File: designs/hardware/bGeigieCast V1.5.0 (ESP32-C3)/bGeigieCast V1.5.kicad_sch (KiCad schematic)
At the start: 9 parts, among them SW1 TACT-SWITCH, SW2 SWITCH_INV, U1 ESP32S, U2 XBEE-socket

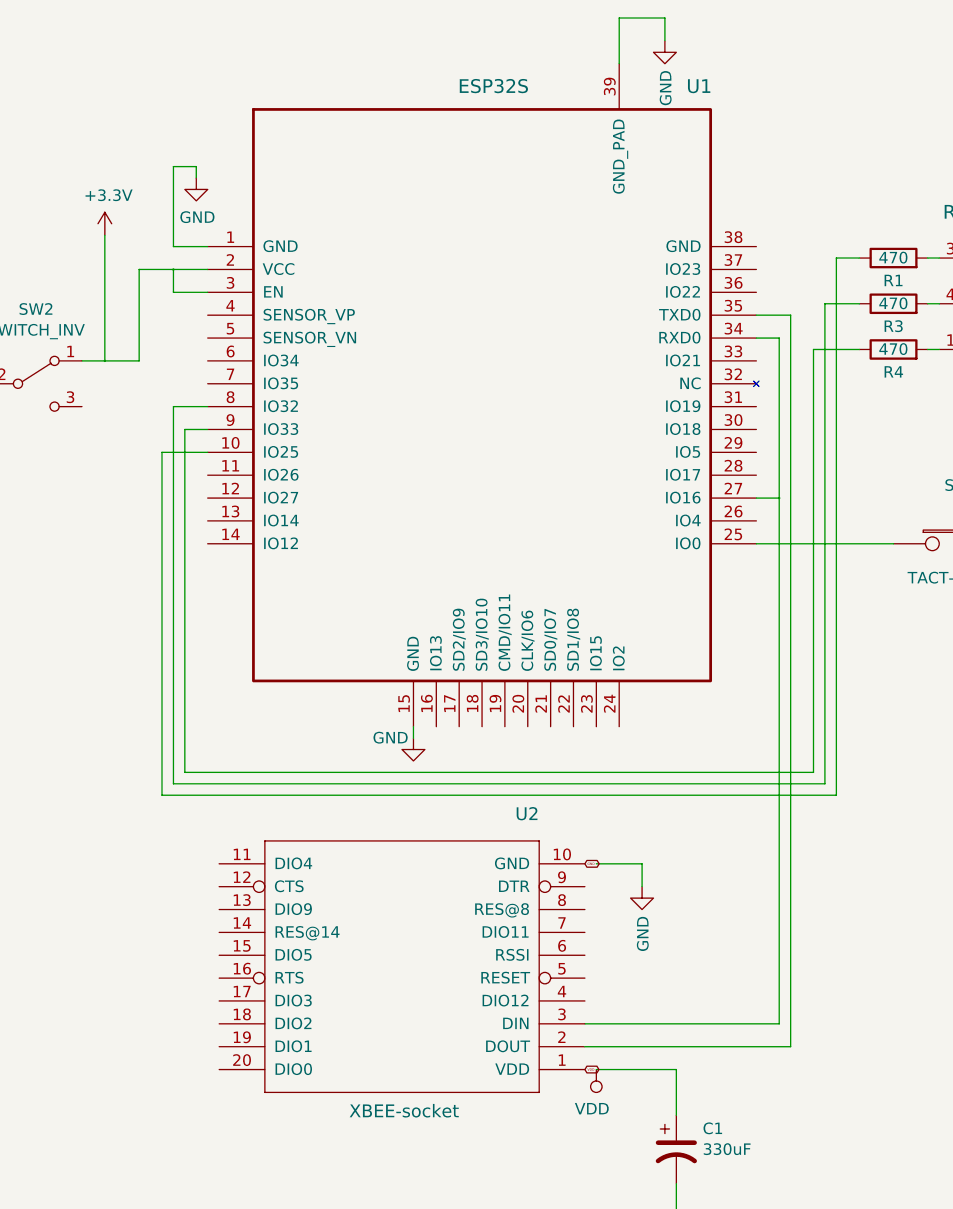
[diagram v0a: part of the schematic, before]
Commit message: V1.5.0 with ESP32-C3
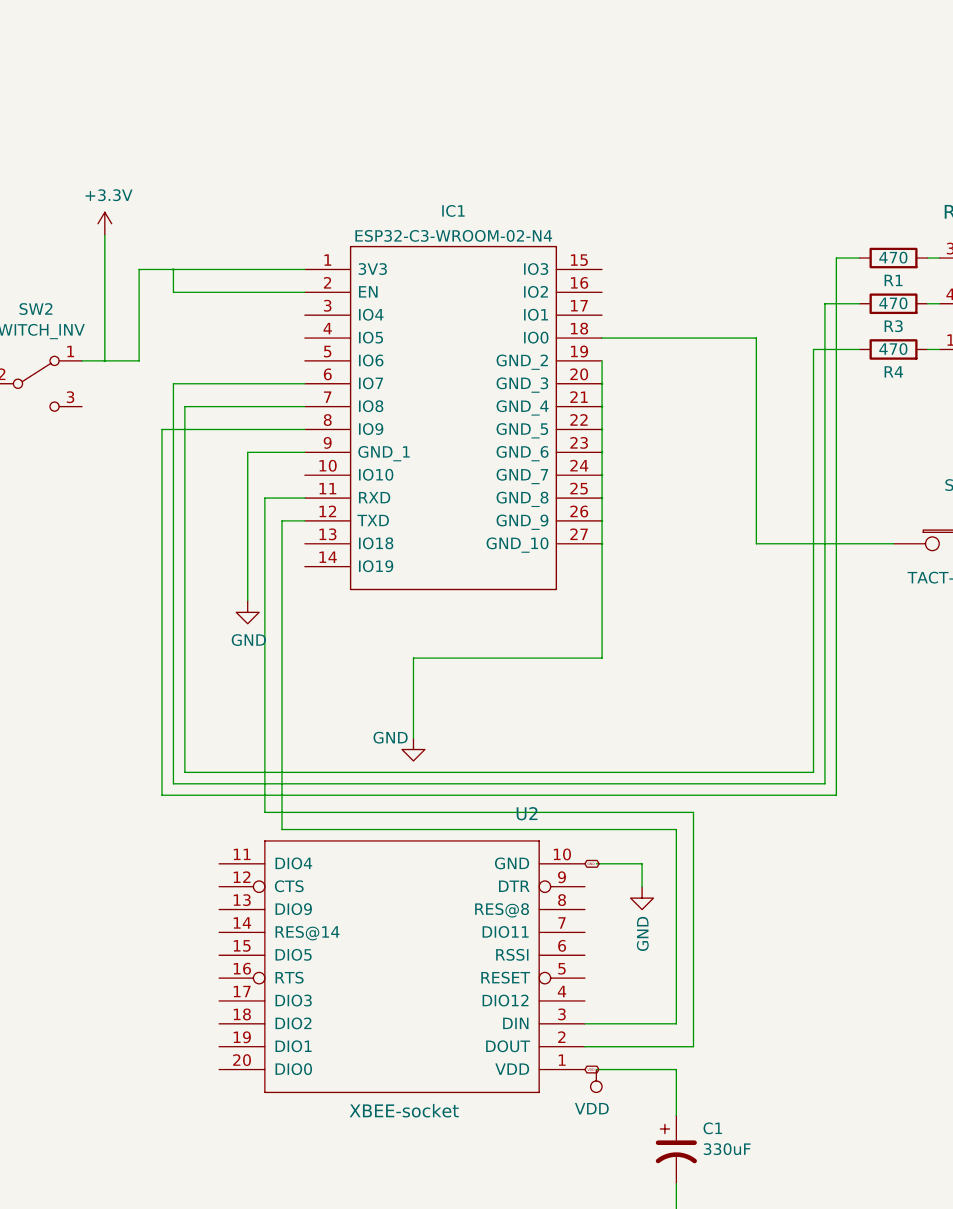
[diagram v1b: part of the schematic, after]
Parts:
- removed U1: ESP32S, ESP32-footprints-Lib:ESP-32S, symbol xbee-rescue:ESP32S-espressif-xess
- added IC1: ESP32-C3-WROOM-02-N4, ESP32C3WROOM02N4, symbol ESP32-C3-WROOM-02-N4:ESP32-C3-WROOM-02-N4
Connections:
- net +3V3: now also IC1.1 (3V3), IC1.2 (EN)
- net GND: now also IC1.19 (GND_2), IC1.20 (GND_3), IC1.21 (GND_4), IC1.22 (GND_5), IC1.23 (GND_6), IC1.24 (GND_7), IC1.25 (GND_8), IC1.26 (GND_9), IC1.27 (GND_10), IC1.9 (GND_1)
- net at U2.2 (DOUT): now also IC1.11 (RXD)
- net at U2.3 (DIN): now also IC1.12 (TXD)
- net at SW1.1: now also IC1.18 (IO0)
- net at R1.1: now also IC1.8 (IO9)
- net at R3.1: now also IC1.6 (IO7)
- net at R4.1: now also IC1.7 (IO8)
